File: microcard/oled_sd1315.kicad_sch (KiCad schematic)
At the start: 13 parts, among them J4 OLED_SSD1315

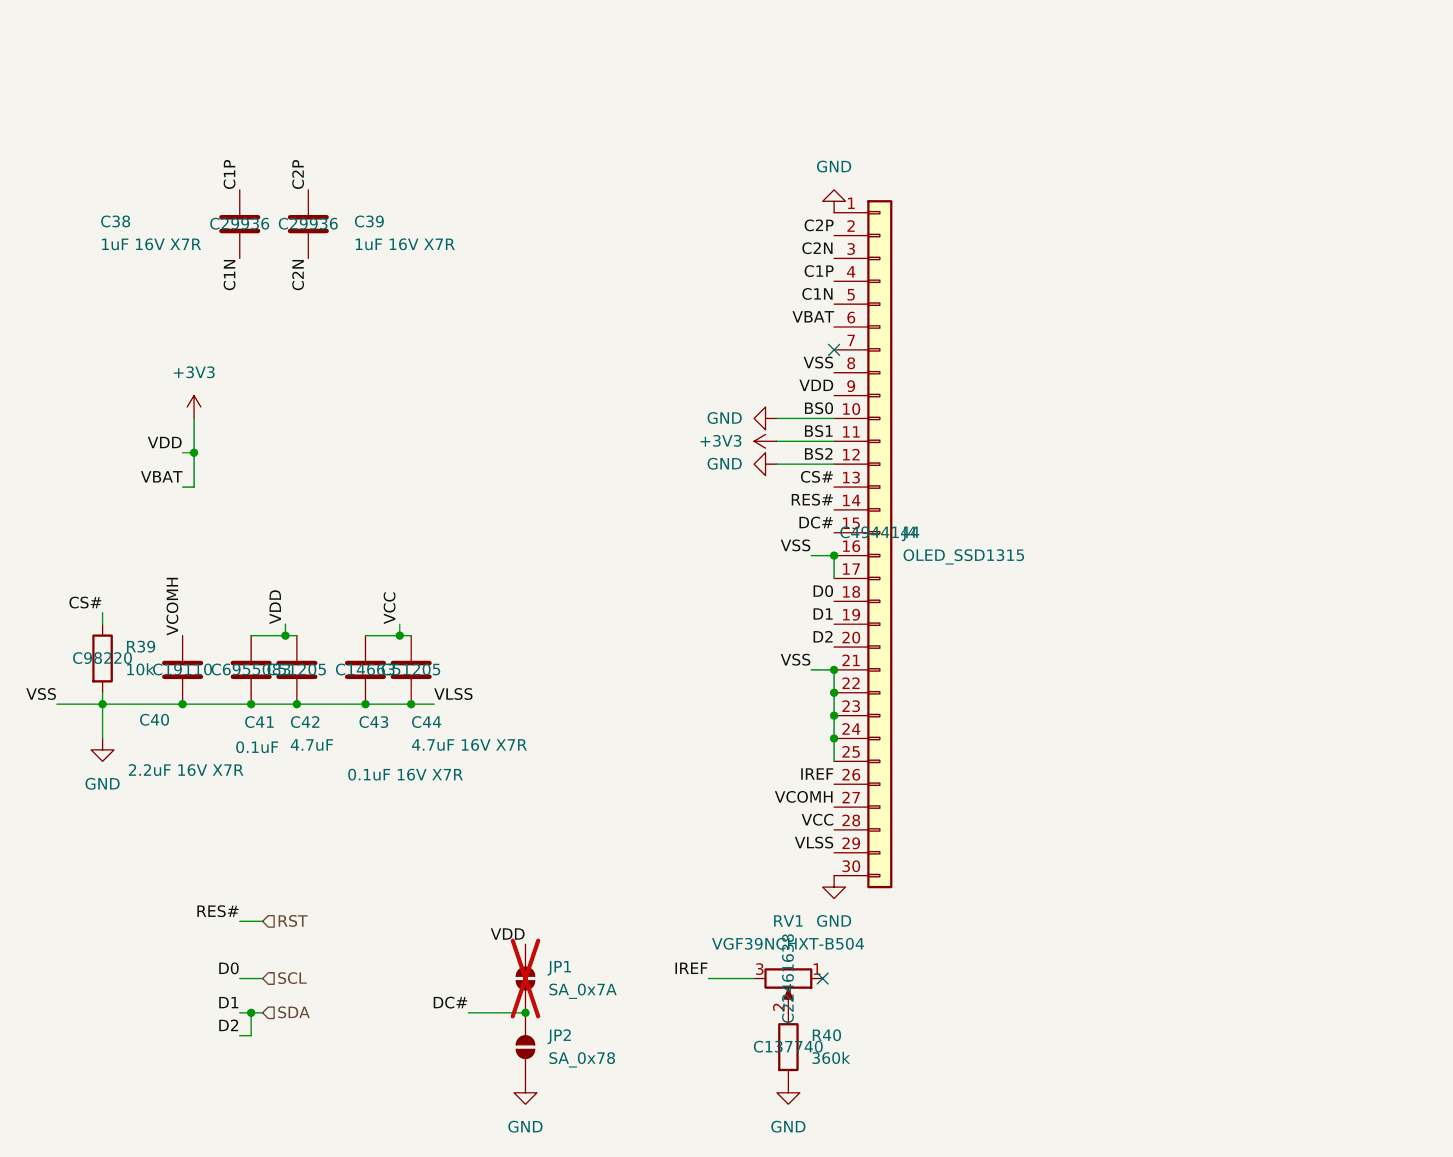
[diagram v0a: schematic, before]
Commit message: wide render
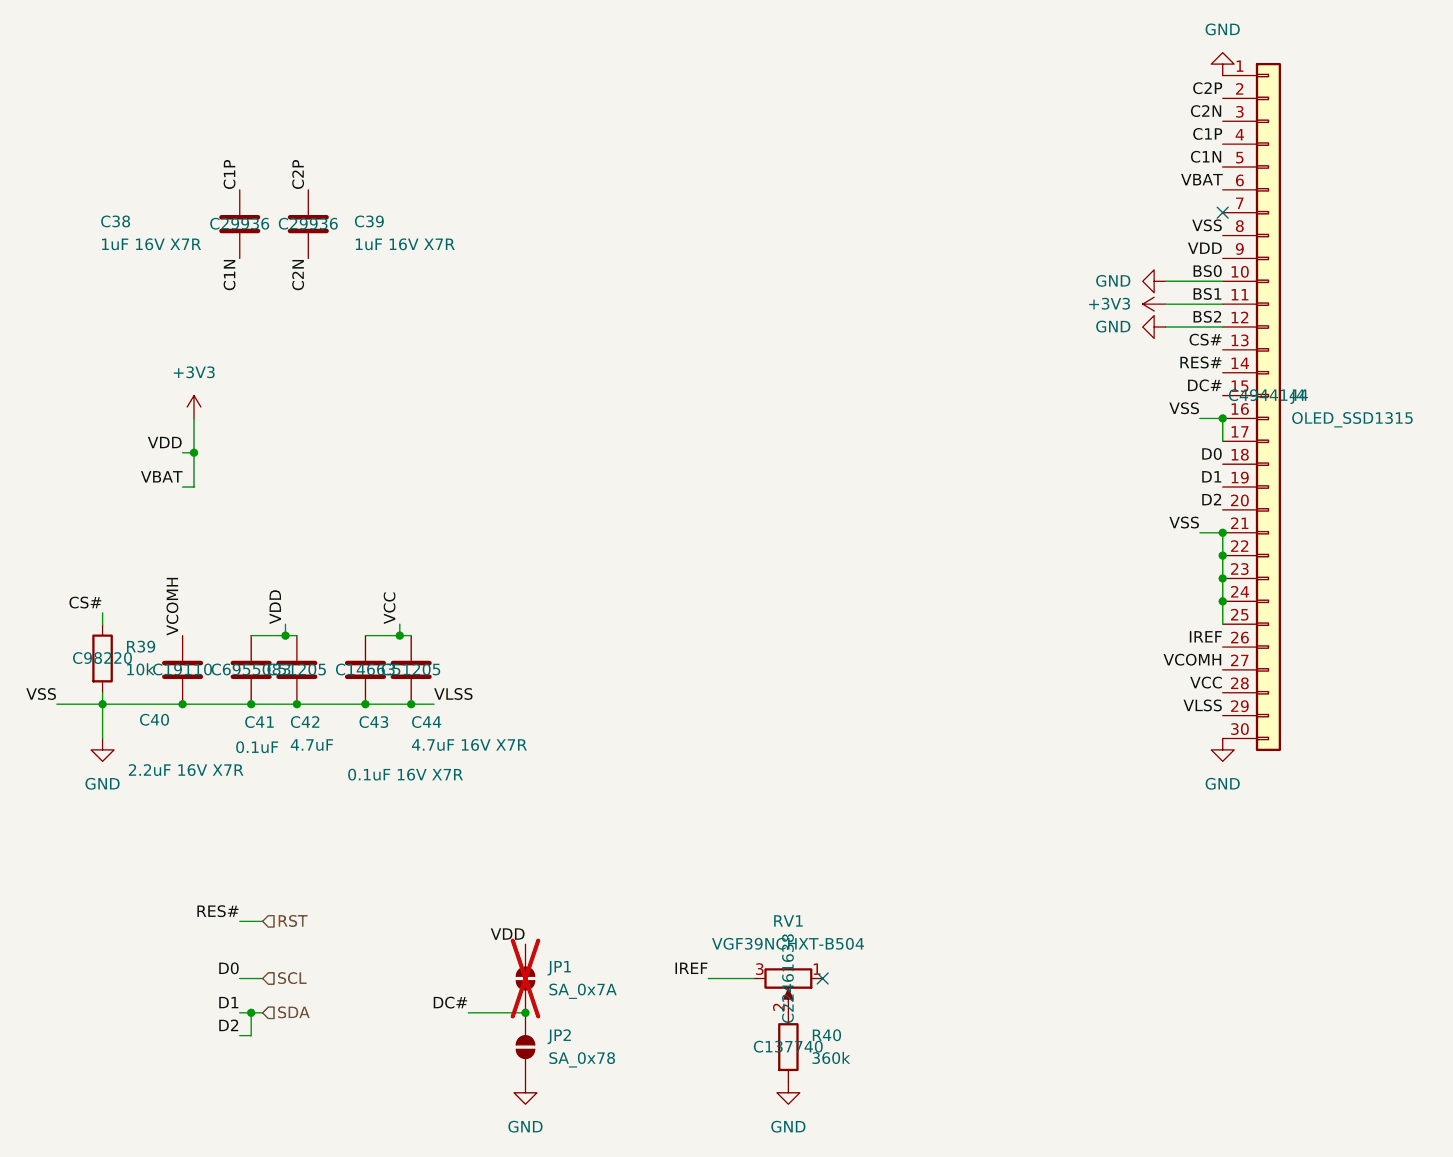
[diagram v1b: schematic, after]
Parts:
- C38, C39, C41, C43: footprint Capacitor_SMD:C_0603_1608Metric_Pad1.08x0.95mm_HandSolder -> Capacitor_SMD:C_0603_1608Metric
- C40: footprint Capacitor_SMD:C_0805_2012Metric_Pad1.18x1.45mm_HandSolder -> Capacitor_SMD:C_0805_2012Metric
- C42, C44: footprint Capacitor_SMD:C_1206_3216Metric_Pad1.33x1.80mm_HandSolder -> Capacitor_SMD:C_1206_3216Metric
- R39, R40: footprint Resistor_SMD:R_0603_1608Metric_Pad0.98x0.95mm_HandSolder -> Resistor_SMD:R_0603_1608Metric
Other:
- moved on the sheet: J4
